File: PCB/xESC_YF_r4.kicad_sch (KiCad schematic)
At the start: 35 parts, among them J1 Conn_01x09_Male, J10 OM-MB W => MC BRK, J11 Conn_01x04_Pin, J2 Conn_01x02_Pin, J3 Conn_01x05_Male, J4 Conn_01x05_Male, J6 OM-MB U => MC SA, J7 Conn_01x06_Male, J8 Conn_01x06_Pin, J9 OM-MB V => MC +24V, U1 STM32C011F6Px, U2 TPS1H200A-Q1, U3 INA139NA, U5 XC6220B331MR

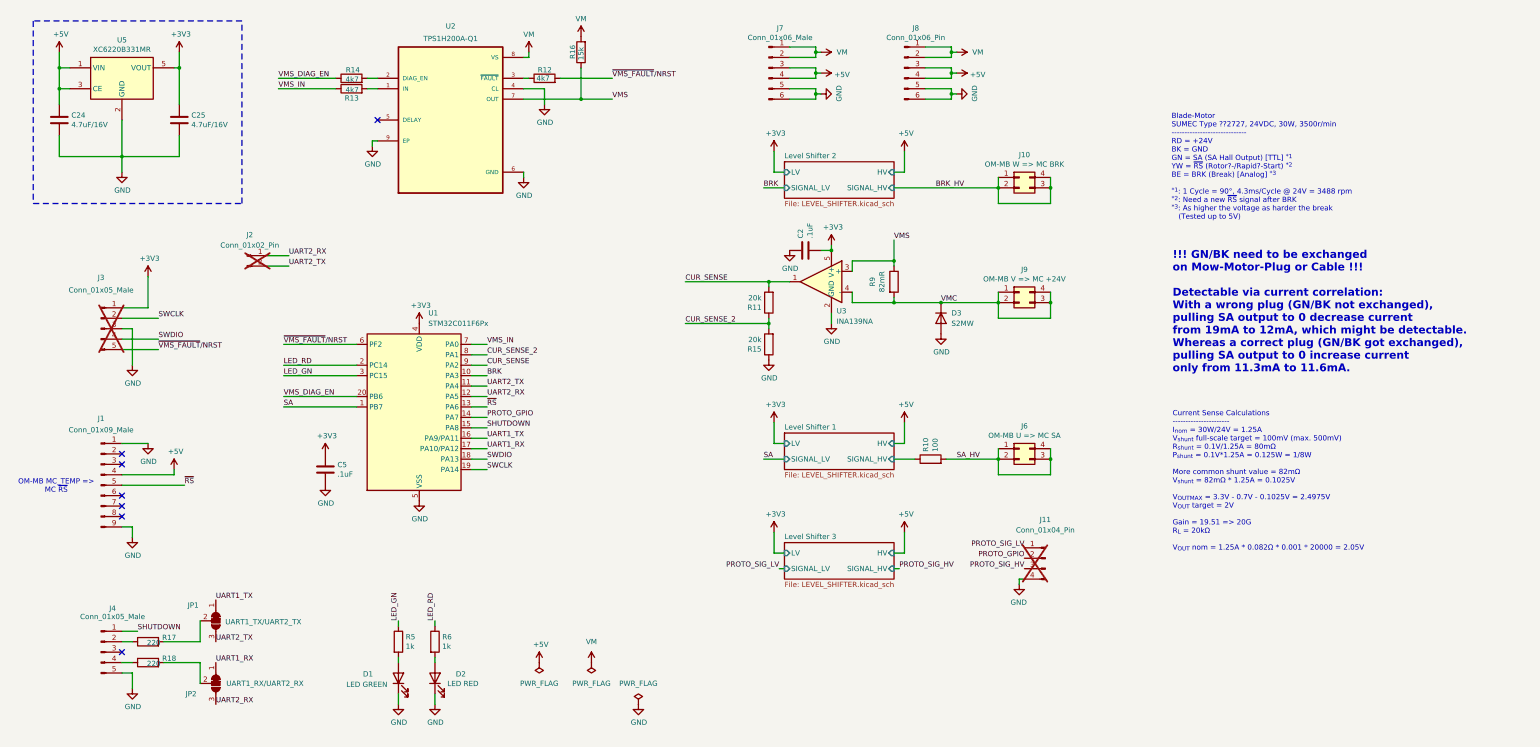
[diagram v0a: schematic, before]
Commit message: Cleanup
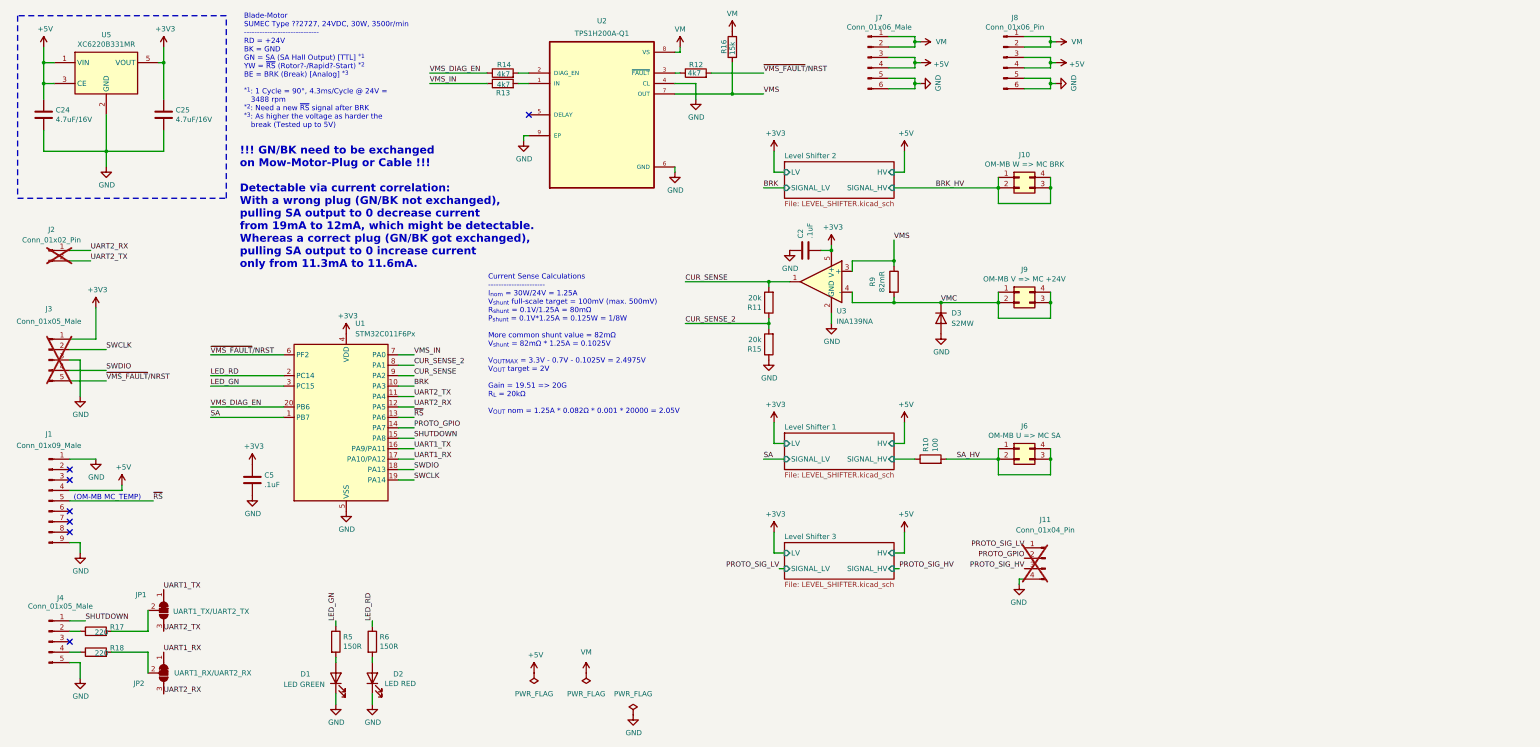
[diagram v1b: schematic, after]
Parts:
- R5, R6: value 1k -> 150R
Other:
- note added: "(OM-MB MC_TEMP)"
- note removed: "OM-MB MC_TEMP => MC ~{RS}"
- moved on the sheet: C24, C25, C5, D1, D2, J1, J2, J3, J4, J7, J8, JP1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
